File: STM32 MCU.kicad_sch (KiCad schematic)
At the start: 33 parts, among them J11 Conn_01x04_Socket, J4 Conn_01x04_Pin, J5 Conn_01x02_Pin, SW2 SW_Push, SW5 SW_Push, U3 STM32G474RETx, Y1 16MHz

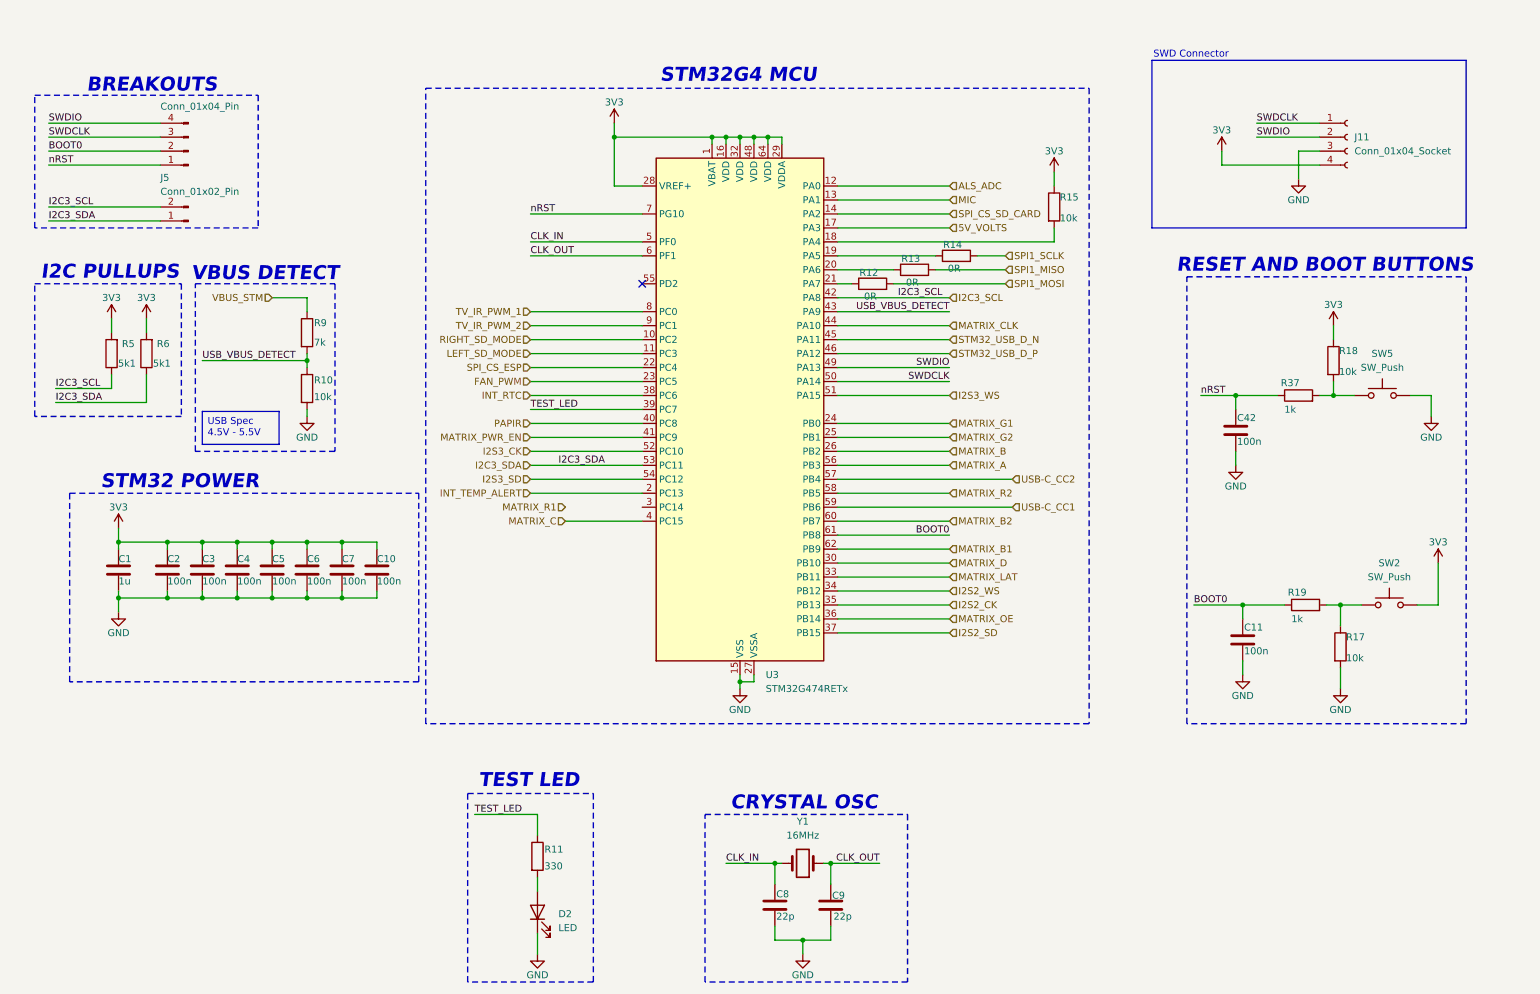
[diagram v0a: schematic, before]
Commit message: Schematic formating
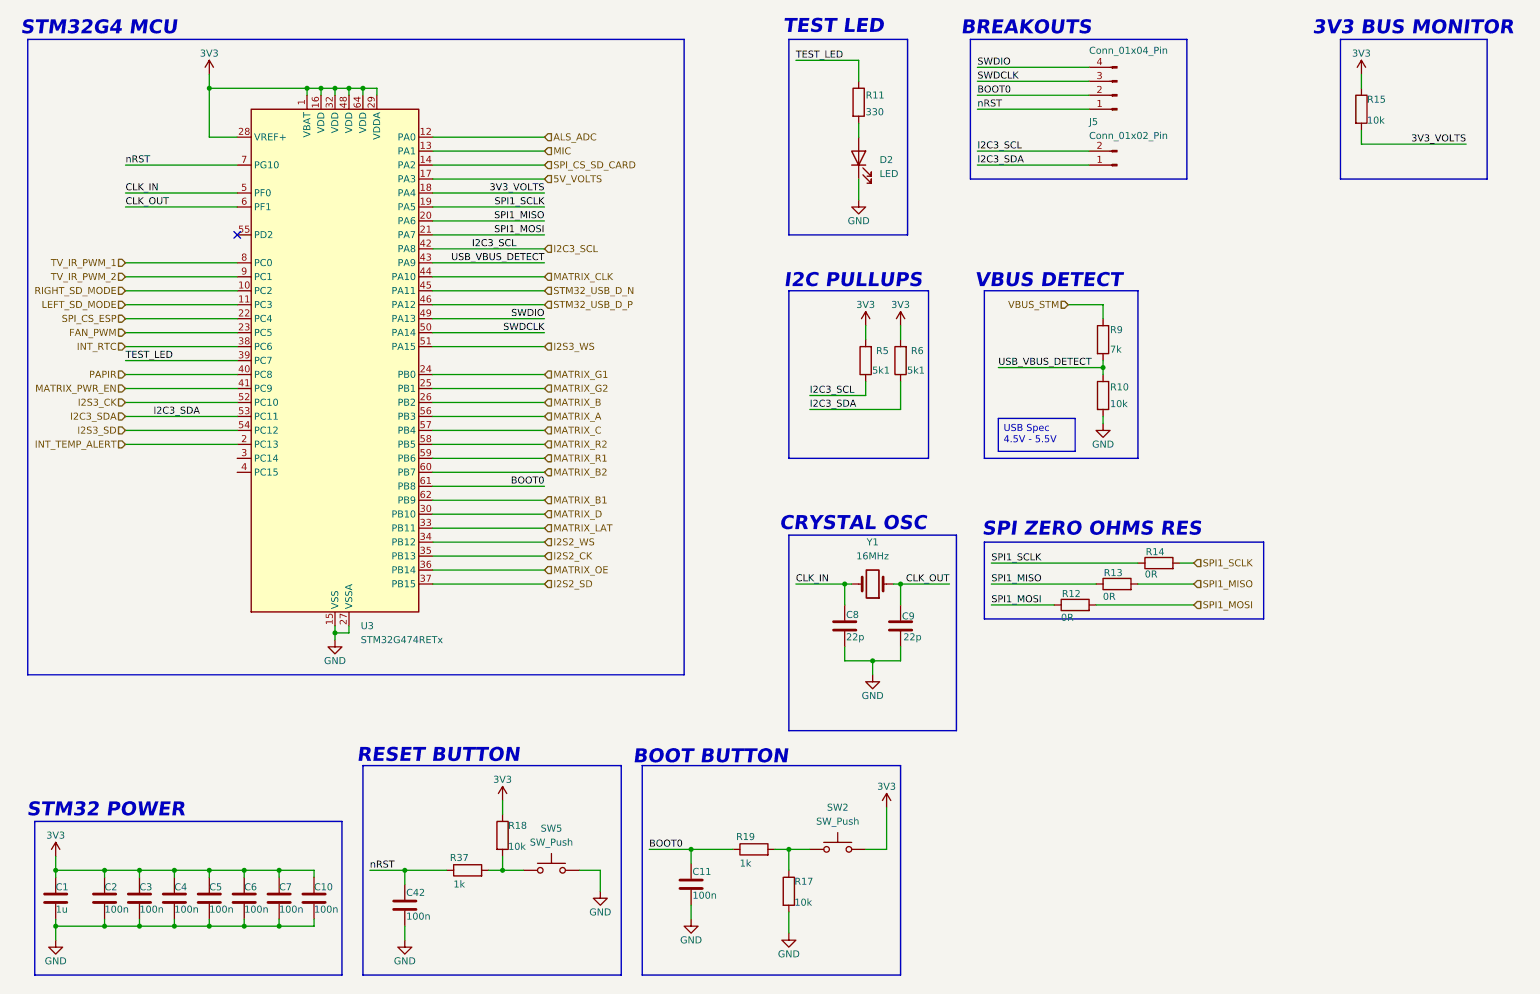
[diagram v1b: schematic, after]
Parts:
- removed J11: Conn_01x04_Socket, Connector_Molex:Molex_SL_171971-0004_1x04_P2.54mm_Vertical, symbol Connector:Conn_01x04_Socket
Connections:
- net USB-C_CC1 is gone; now on net MATRIX_R1: U3.59 (PB6)
- net USB-C_CC2 is gone; now on net MATRIX_C: U3.57 (PB4)
- net MATRIX_C: no longer U3.4 (PC15)
- net SPI1_MISO: now also R13.1, U3.20 (PA6)
- net SPI1_MOSI: now also R12.1, U3.21 (PA7)
- net SPI1_SCLK: now also R14.1, U3.19 (PA5)
- net 3V3_VOLTS: now reaches R15.2, U3.18 (PA4)
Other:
- note added: "3V3 BUS MONITOR"
- note added: "BOOT BUTTON"
- note added: "RESET BUTTON"
- note added: "SPI ZERO OHMS RES"
- note removed: "RESET AND BOOT BUTTONS"
- note removed: "SWD Connector"
- moved on the sheet: C1, C10, C11, C2, C3, C4, C42, C5, C6, C7, C8, C9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
